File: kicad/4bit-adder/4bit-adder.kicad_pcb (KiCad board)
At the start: 2 copper layers, 98 parts, among them J1 Screw_Terminal_01x02, K1 SR11-5V-200-2C-PH, K10 SR11-5V-200-2C-PH, K11 SR11-5V-200-2C-PH, K12 SR11-5V-200-2C-PH, K13 SR11-5V-200-2C-PH, K14 SR11-5V-200-2C-PH, K15 SR11-5V-200-2C-PH, K16 SR11-5V-200-2C-PH, K17 SR11-5V-200-2C-PH, K18 SR11-5V-200-2C-PH, K19 SR11-5V-200-2C-PH, K2 SR11-5V-200-2C-PH, K20 SR11-5V-200-2C-PH, K21 SR11-5V-200-2C-PH, K22 SR11-5V-200-2C-PH, K23 SR11-5V-200-2C-PH, K24 SR11-5V-200-2C-PH, K3 SR11-5V-200-2C-PH, K4 SR11-5V-200-2C-PH, K5 SR11-5V-200-2C-PH, K6 SR11-5V-200-2C-PH, K7 SR11-5V-200-2C-PH, K8 SR11-5V-200-2C-PH, K9 SR11-5V-200-2C-PH, SW1 SW_Wuerth_450301014042, SW3 A, SW4 B

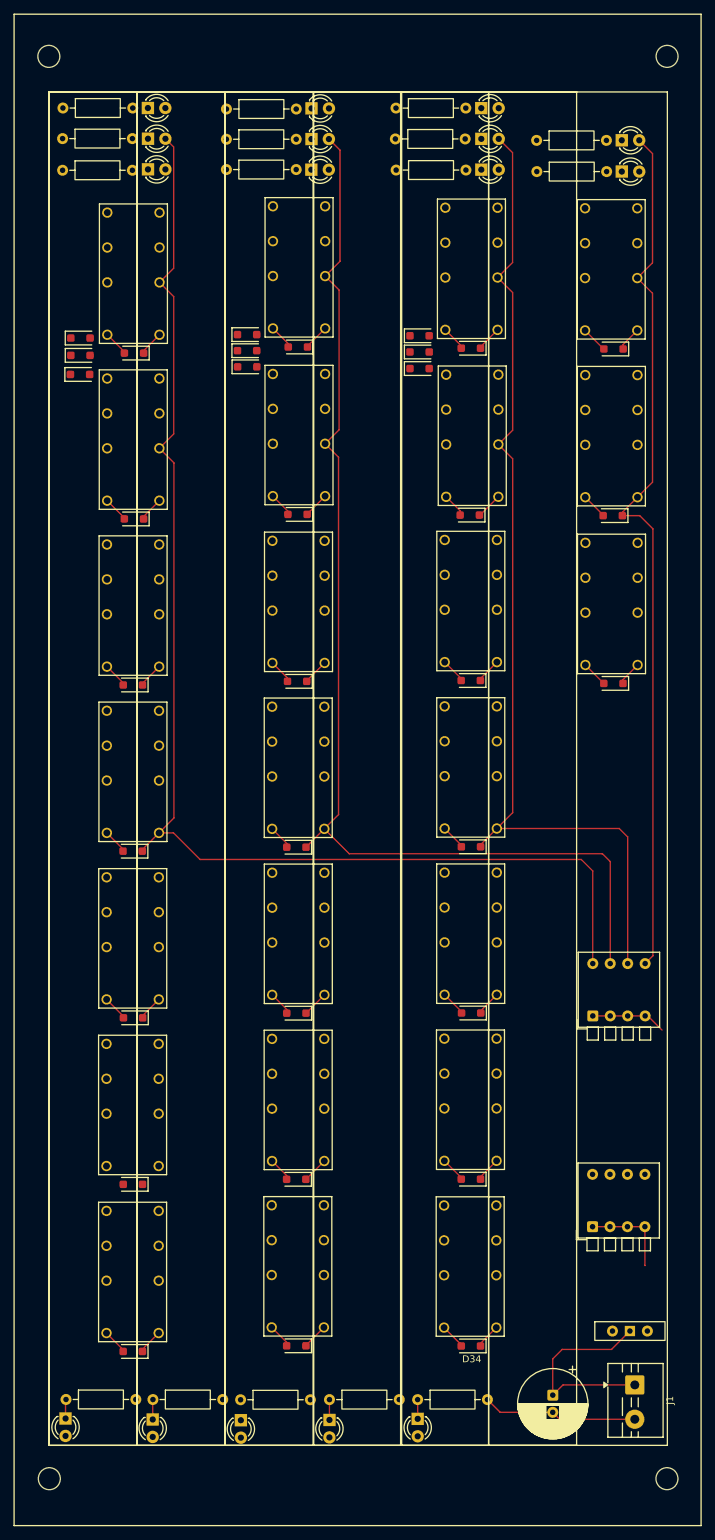
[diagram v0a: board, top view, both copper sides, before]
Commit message: finished pcb wiring
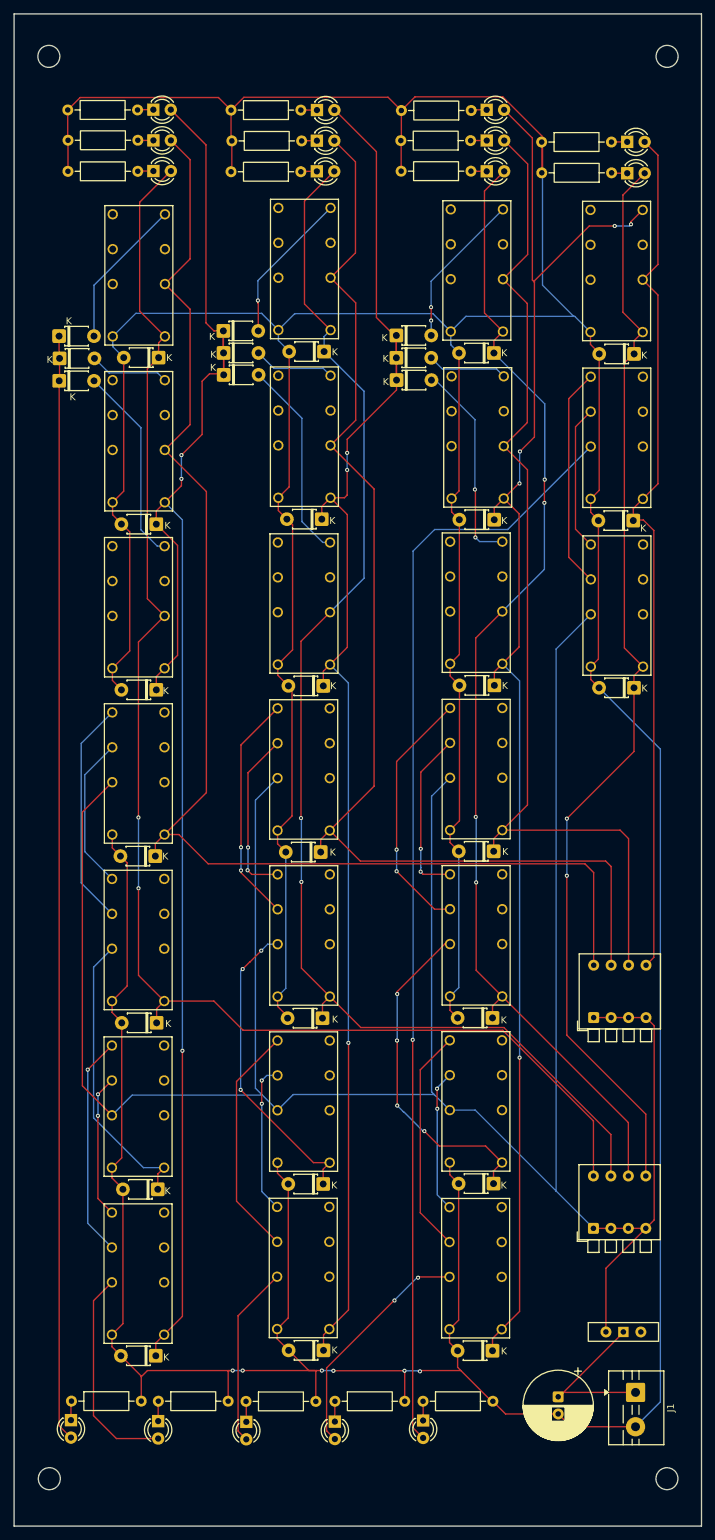
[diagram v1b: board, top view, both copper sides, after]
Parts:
- D1, D22, D23, D24, D26, D27, D28, D29, D3, D30, D31, D32, D33, D34, D35, D36, D37, D38, D39, D4, D40, D41, D42, D43, D44, D45, D46, D47, D48, D49, D5, D6, D7: footprint Diode_SMD:D_SOD-123F -> Diode_THT:D_T-1_P5.08mm_Horizontal
- moved R10 11.0 mm to (68.1, 31.5), turned to 180 degrees
- moved R16 11.0 mm to (91.9, 31.6), turned to 180 degrees
- moved R18 11.0 mm to (116.5, 31.5), turned to 180 degrees
- moved R20 10.9 mm to (116.6, 27.1), turned to 180 degrees
- moved R15 10.9 mm to (68.0, 36.0), turned to 180 degrees
- moved R19 10.9 mm to (116.5, 36.0), turned to 180 degrees
- moved R21 10.9 mm to (137.0, 36.2), turned to 180 degrees
- moved R23 10.9 mm to (68.0, 27.1), turned to 180 degrees
- moved R17 10.8 mm to (91.8, 36.1), turned to 180 degrees
- moved R22 10.8 mm to (91.8, 27.1), turned to 180 degrees
- moved D35 4.01 mm to (95.1, 207.6)
- moved D38 3.98 mm to (95.0, 183.4)
- moved D48 3.87 mm to (95.2, 62.2)
- moved D39 3.87 mm to (94.9, 159.3)
- moved D44 3.87 mm to (95.1, 110.9)
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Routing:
- net GND: track 106.6 -> 888.4 mm, vias 0 -> 6
- net SWV: track 24.2 -> 379.4 mm
- net Net-(D12-A): track 11.0 -> 229.7 mm, vias 0 -> 3
- net Net-(D30-K): track 11.2 -> 216.7 mm, vias 0 -> 5
- net Net-(D15-A): track 7.28 -> 210.7 mm, vias 0 -> 2
- net Net-(D1-K): track 11.3 -> 208.4 mm, vias 0 -> 3
- net Net-(D17-A): track 7.55 -> 190.4 mm, vias 0 -> 2
- net Net-(D19-A): track 7.32 -> 169.2 mm, vias 0 -> 4
- net Net-(D8-A): track 0.00 -> 161.9 mm, vias 0 -> 1
- net Net-(D22-K): track 0.00 -> 161.1 mm
- net Net-(D21-A): track 7.11 -> 160.1 mm, vias 0 -> 2
- net Net-(D49-K): track 3.64 -> 49.6 mm, vias 0 -> 4
- net Net-(D37-K): track 0.00 -> 42.5 mm
- net Net-(D38-K): track 3.78 -> 45.1 mm, vias 0 -> 3
- net Net-(K4-PadNO2): track 0.00 -> 37.0 mm, vias 0 -> 2
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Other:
- board outline added: 100.1 x 220.1 mm
